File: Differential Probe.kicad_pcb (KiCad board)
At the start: 4 copper layers, 115 x 60 mm, 113 parts, among them J1 Conn_01x01_Pin, J2 Conn_01x01_Pin, J3 USB_C_Receptacle_PowerOnly_6P, J4 Conn_Coaxial, SW2 SW_DIP_x03, U1 BQ24072RGT, U2 OPA810xD, U3 OPA810xD, U4 OPA810xD, U5 TPS65135RTER

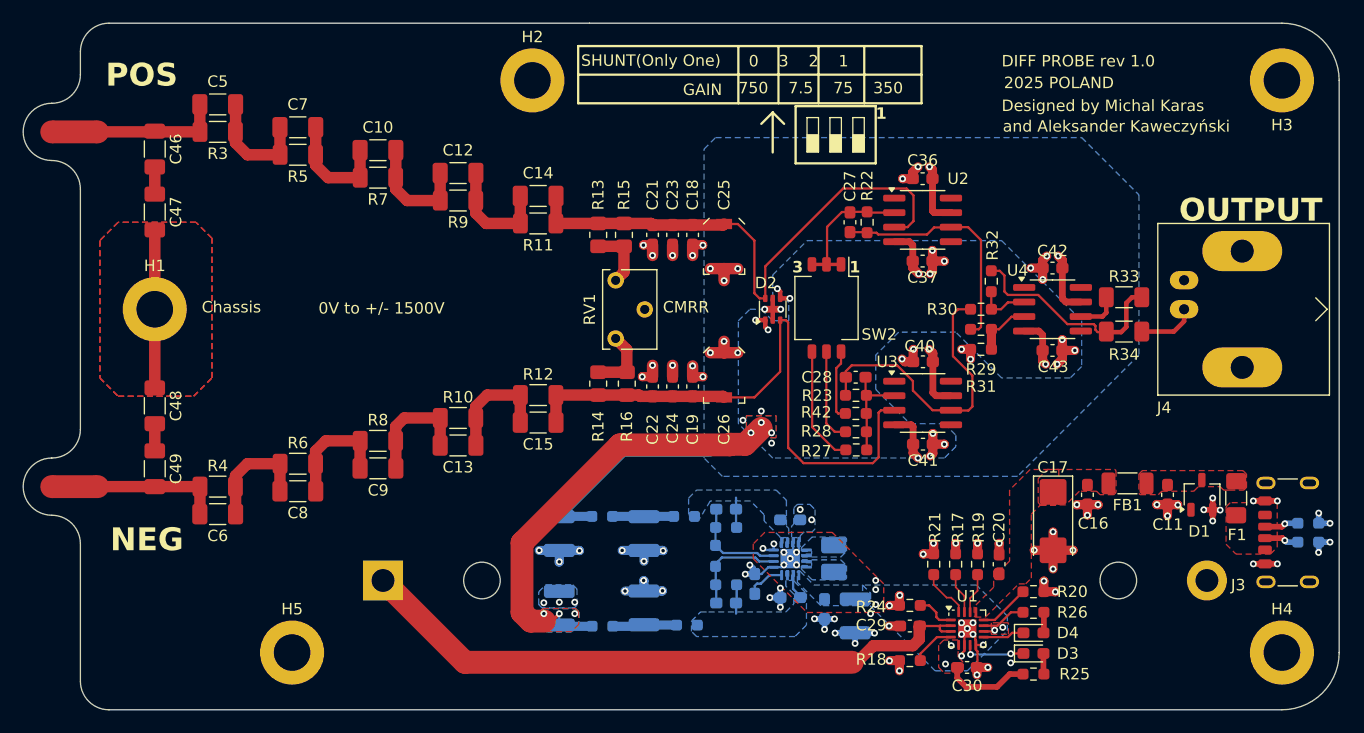
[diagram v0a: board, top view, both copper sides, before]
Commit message: Done
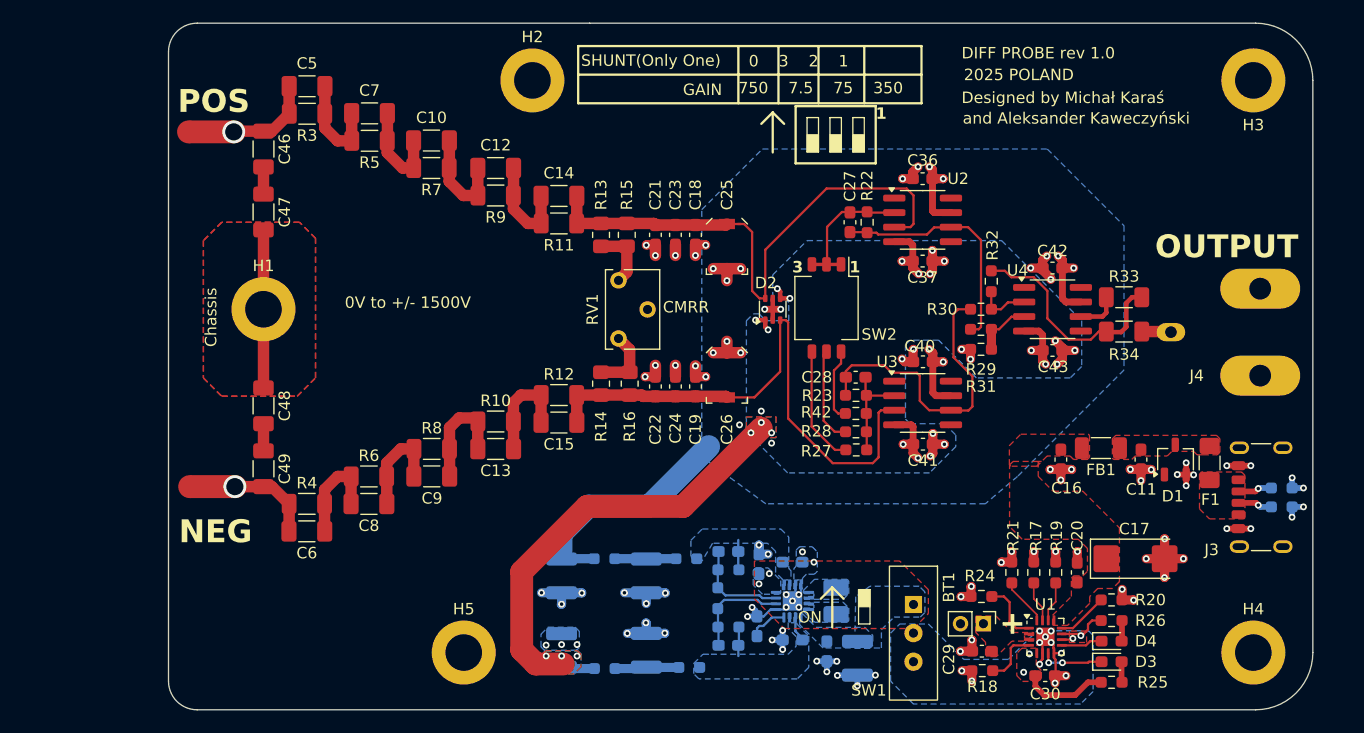
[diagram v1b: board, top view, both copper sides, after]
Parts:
- added C52: 100n, Capacitor_SMD:C_0603_1608Metric_Pad1.08x0.95mm_HandSolder, B.Cu at (138.3, 138.8)
- added SW1: EG1218, Button_Switch_THT:SW_Slide-03_Wuerth-WS-SLTV_10x2.5x6.4_P2.54mm, F.Cu at (151.8, 144.8)
- BT1: value 18650 -> LiPo; footprint Battery:BatteryHolder_MPD_BH-18650-PC2 -> Connector_PinHeader_2.00mm:PinHeader_1x02_P2.00mm_Vertical; moved to F.Cu
- J4: footprint Connector_Coaxial:BNC_Amphenol_B6252HB-NPP3G-50_Horizontal -> Library:BNC_Molex_73100-0154-50_Horizontal
- moved BT1 52.6 mm to (157.9, 144.0), turned to -90 degrees
- moved H5 15.0 mm to (112.5, 146.5)
- moved J2 12.0 mm to (90.5, 132.0)
- moved J1 12.0 mm to (90.5, 101.0)
- moved C46 9.50 mm to (95.0, 102.5)
- moved C47 9.50 mm to (95.0, 108.0)
- moved C48 9.50 mm to (95.0, 124.9)
- moved C49 9.50 mm to (95.0, 130.4)
- moved H1 9.50 mm to (95.0, 116.5)
- moved C5 7.96 mm to (98.8, 97.0)
- moved R3 7.96 mm to (98.8, 99.4)
- moved C6 7.93 mm to (98.8, 135.9)
- moved R4 7.93 mm to (98.8, 133.5)
- moved C17 7.92 mm to (171.2, 138.3), turned to 0 degrees
- moved C20 6.87 mm to (166.1, 139.5)
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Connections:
- C31 pad 1: OUT -> Net-(SW1-B)
- C32 pad 1: OUT -> Net-(SW1-B)
- U5 pad 1: OUT -> Net-(SW1-B)
- U5 pad 8: OUT -> Net-(SW1-B)
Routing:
- net Net-(BT1-+): track 55.9 -> 0.00 mm
- net -6V: track 56.0 -> 60.9 mm, vias 13 -> 16
- net +6V: track 38.5 -> 43.4 mm, vias 5 -> 8
- net GND: track 110.5 -> 114.3 mm
- net Net-(J2-Pin_1): track 11.4 -> 7.72 mm, vias 0 -> 1
- net Net-(D2B-K1A2): track 53.3 -> 50.2 mm
- net Net-(J4-In): track 5.12 -> 2.80 mm
- net Net-(U1-TS): track 3.43 -> 5.38 mm
- net Net-(C10-Pad2): track 10.1 -> 8.72 mm
- net Net-(C8-Pad2): track 10.2 -> 8.89 mm
- net Net-(C12-Pad1): track 10.2 -> 8.94 mm
- net Net-(C6-Pad2): track 10.1 -> 8.86 mm
- net Net-(C5-Pad1): track 10.1 -> 8.88 mm
- net Net-(C10-Pad1): track 10.1 -> 9.00 mm
- net Net-(U1-~{CE}): track 3.86 -> 4.90 mm
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- added copper zone on F.Cu, net Net-(BT1-+)
- added copper zone on B.Cu, net Net-(SW1-B)
- added copper zone on F.Cu, net Net-(SW1-B)
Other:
- board size 115 x 60 mm -> 100 x 60 mm
- board text added: "+"
- board text added: "Designed by Michał Karaś"
- board text added: "ON"
- board text removed: "Designed by Michal Karas"
